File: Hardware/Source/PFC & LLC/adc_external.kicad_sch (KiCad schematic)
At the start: 9 parts, among them U8 ADS1115IDGS

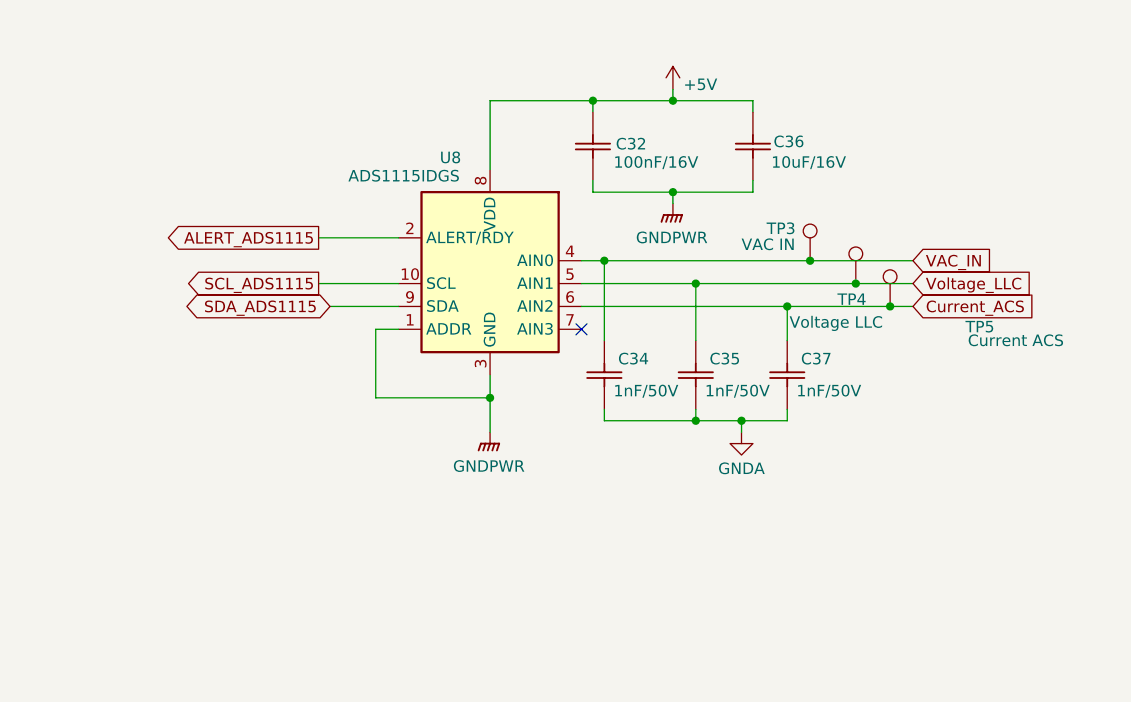
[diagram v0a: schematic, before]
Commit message: update FEEDBACK, AC
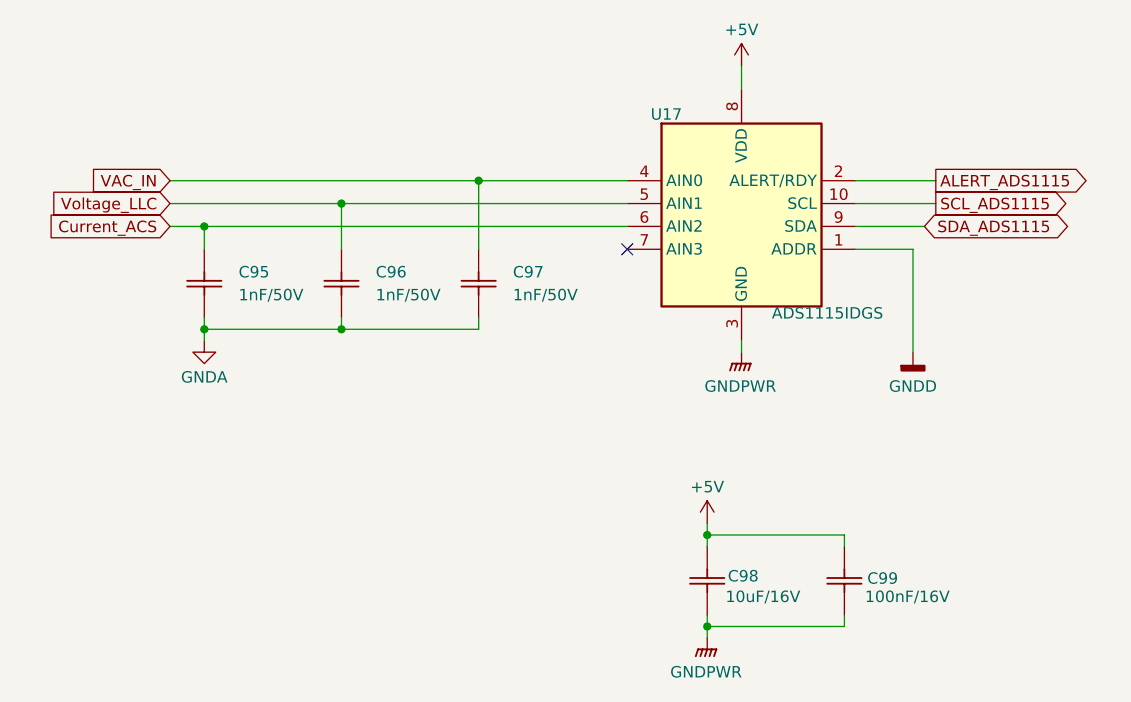
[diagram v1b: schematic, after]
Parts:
- removed C32: 100nF/16V, charge_battery_footprint_lib:Ceramic_Cap_0603, symbol charge_battery_sym_lib:Ceramic_Cap_SMD_100nF_16V
- removed C34, C35, C37: 1nF/50V, charge_battery_footprint_lib:Ceramic_Cap_0603, symbol charge_battery_sym_lib:Ceramic_Cap_SMD_1nF_50V
- removed C36: 10uF/16V, charge_battery_footprint_lib:Ceramic_Cap_0603, symbol charge_battery_sym_lib:Ceramic_Cap_SMD_10uF_16V
- removed TP3: VAC IN, TestPoint:TestPoint_Bridge_Pitch2.0mm_Drill0.7mm, symbol Connector:TestPoint
- removed TP4: Voltage LLC, TestPoint:TestPoint_Bridge_Pitch2.0mm_Drill0.7mm, symbol Connector:TestPoint
- removed TP5: Current ACS, TestPoint:TestPoint_Bridge_Pitch2.0mm_Drill0.7mm, symbol Connector:TestPoint
- removed U8: ADS1115IDGS, charge_battery_footprint_lib:VSSOP-10, symbol charge_battery_sym_lib:ADS1115IDGS
- added C95, C96, C97: 1nF/50V, charge_battery_footprint_lib:Ceramic_Cap_0603, symbol charge_battery_sym_lib:Ceramic_Cap_SMD_1nF_50V
- added C98: 10uF/16V, charge_battery_footprint_lib:Ceramic_Cap_0603, symbol charge_battery_sym_lib:Ceramic_Cap_SMD_10uF_16V
- added C99: 100nF/16V, charge_battery_footprint_lib:Ceramic_Cap_0603, symbol charge_battery_sym_lib:Ceramic_Cap_SMD_100nF_16V
- added U17: ADS1115IDGS, charge_battery_footprint_lib:VSSOP-10, symbol charge_battery_sym_lib:ADS1115IDGS
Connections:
- net +5V: now also C98.2, C99.2, U17.8 (VDD)
- net ALERT_ADS1115: now also U17.2 (ALERT/RDY)
- net Current_ACS: now also C95.2, U17.6 (AIN2)
- net GNDA: now also C95.1, C96.1, C97.1
- net GNDPWR: now also C98.1, C99.1, U17.3 (GND)
- net SCL_ADS1115: now also U17.10 (SCL)
- net SDA_ADS1115: now also U17.9 (SDA)
- net VAC_IN: now also C97.2, U17.4 (AIN0)
- net Voltage_LLC: now also C96.2, U17.5 (AIN1)
- new net GNDD: U17.1 (ADDR)
